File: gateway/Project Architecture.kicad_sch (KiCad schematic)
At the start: 0 parts

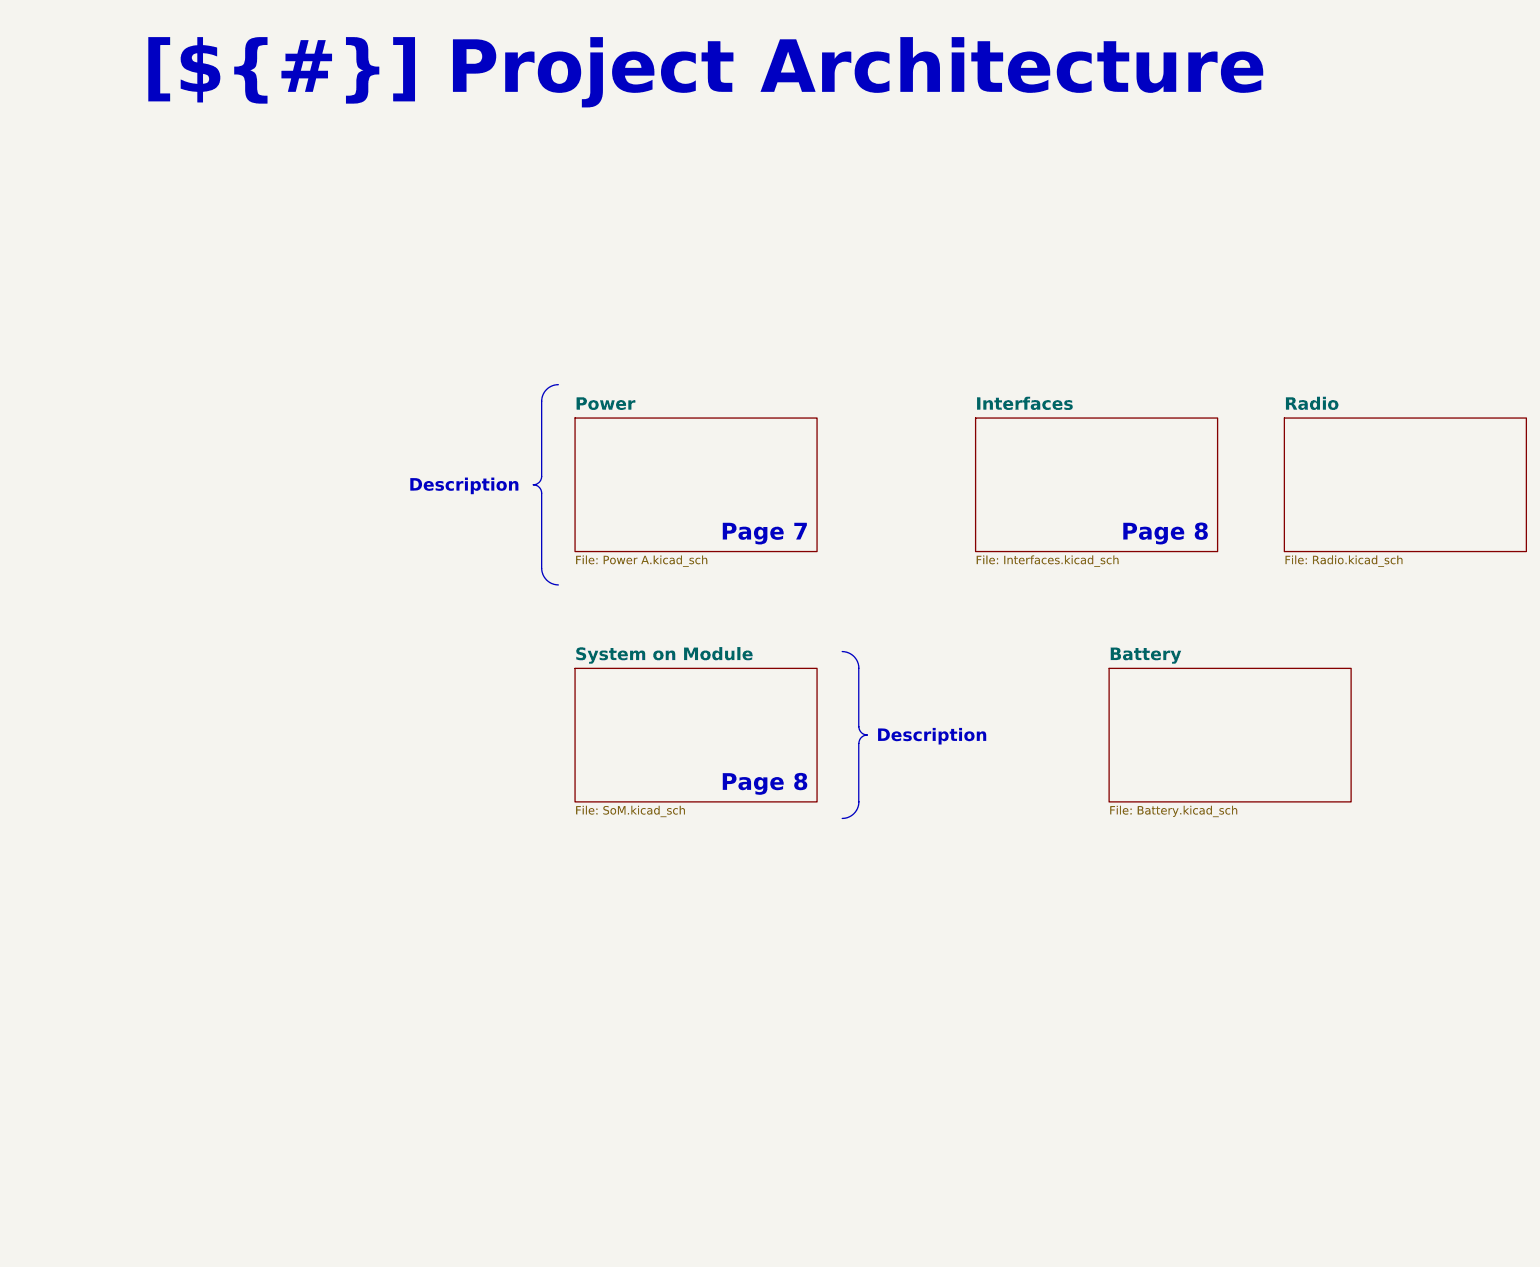
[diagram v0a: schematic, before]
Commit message: Working on first version
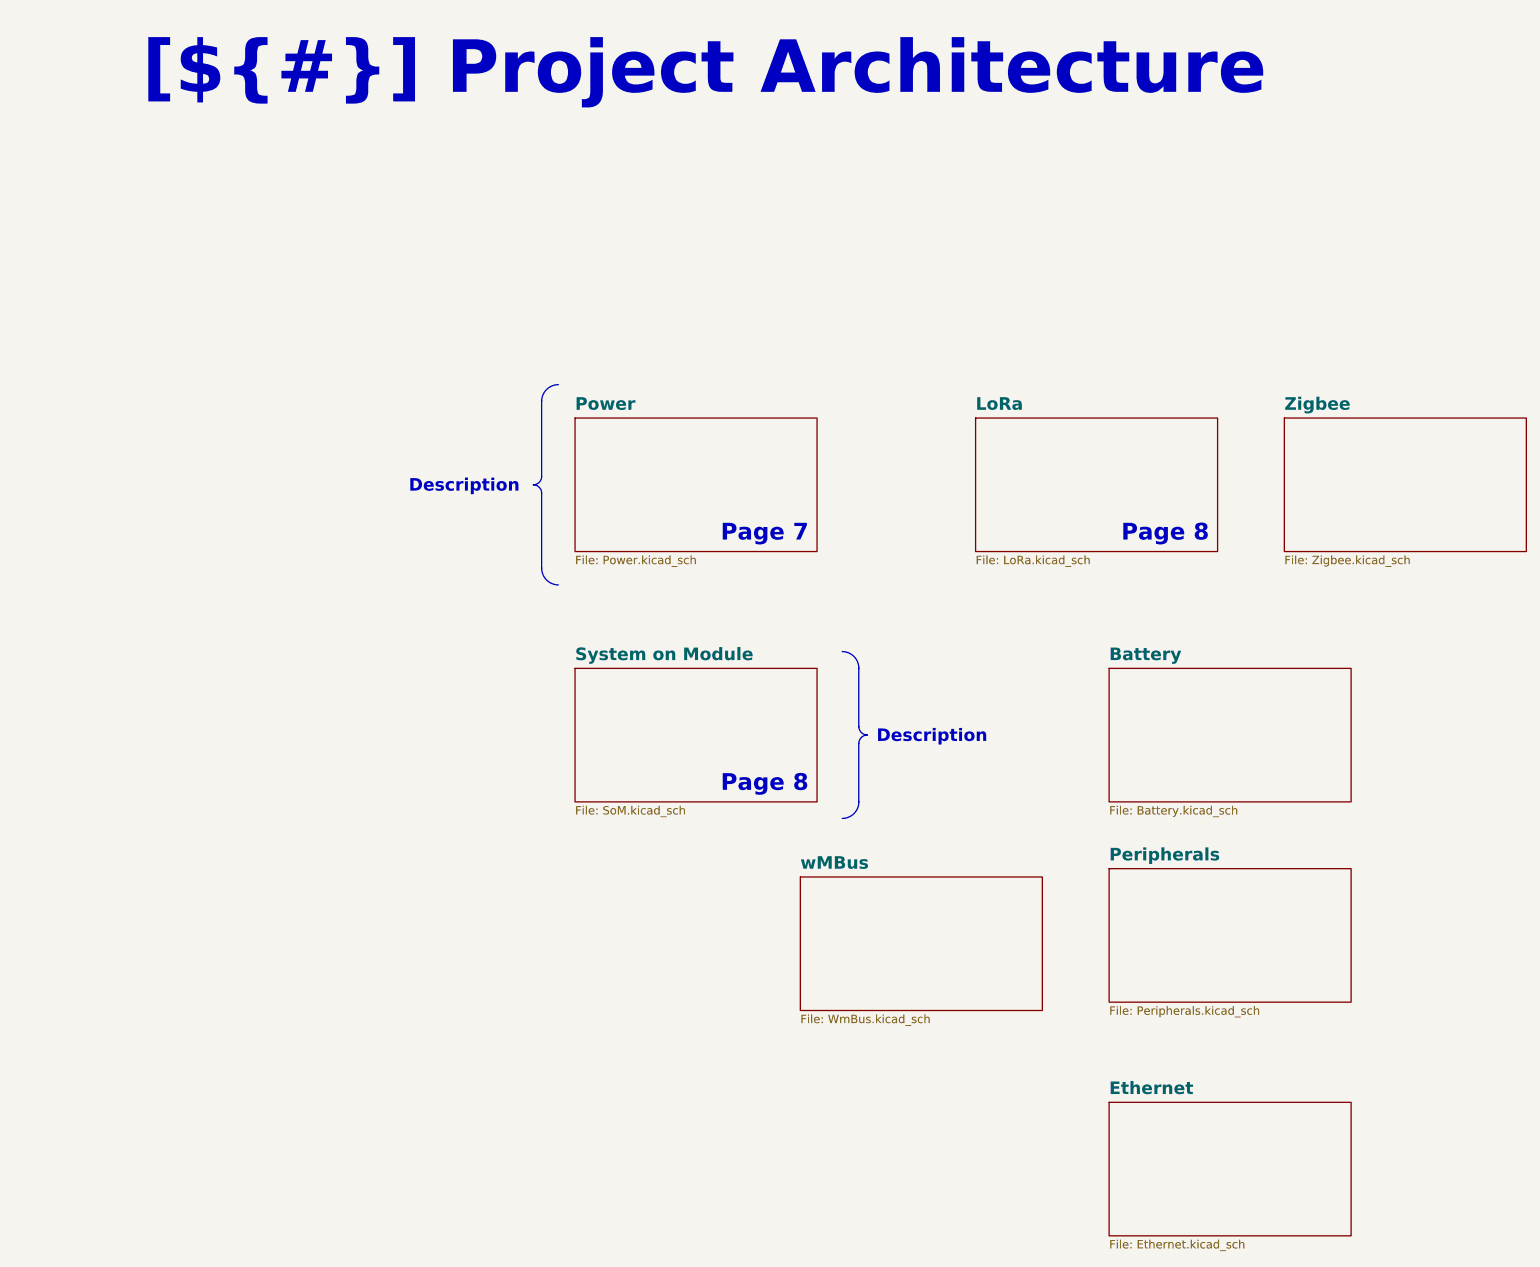
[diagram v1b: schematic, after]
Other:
- sheet Interfaces renamed LoRa
- sheet Radio renamed Zigbee
- added sheet Ethernet (Ethernet.kicad_sch)
- added sheet Peripherals (Peripherals.kicad_sch)
- added sheet wMBus (WmBus.kicad_sch)
- sheet LoRa: file Interfaces.kicad_sch -> LoRa.kicad_sch
- sheet Power: file Power A.kicad_sch -> Power.kicad_sch
- sheet Zigbee: file Radio.kicad_sch -> Zigbee.kicad_sch
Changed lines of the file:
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@@
 			(color 255 200 0 0.502)
 		)
-		(property "Sheetname" "Interfaces"
+		(property "Sheetname" "LoRa"
 			(at 251.46 75.1709 0)
 			(show_name no)
@@
 			)
 		)
-		(property "Sheetfile" "Interfaces.kicad_sch"
+		(property "Sheetfile" "LoRa.kicad_sch"
 			(at 251.46 97.1046 0)
 			(show_name no)
@@
 			(color 255 200 0 0.502)
 		)
-		(property "Sheetname" "Radio"
+		(property "Sheetname" "Zigbee"
 			(at 298.45 75.1709 0)
 			(show_name no)
@@
 			)
 		)
-		(property "Sheetfile" "Radio.kicad_sch"
+		(property "Sheetfile" "Zigbee.kicad_sch"
 			(at 298.45 97.1046 0)
 			(show_name no)
@@
 				(path "/d5742f03-3b1a-42e5-a384-018bd4b919aa/c5103ceb-5325-4a84-a025-9638a412984e"
 					(page "10")
+				)
+			)
+		)
+	)
+	(sheet
+		(at 224.79 146.05)
+		(size 36.83 20.32)
+		(exclude_from_sim no)
+		(in_bom yes)
+		(on_board yes)
+		(dnp no)
+		(fields_autoplaced yes)
+		(stroke
+			(width 0.1524)
+			(type solid)
+		)
+		(fill
+			(color 255 200 0 0.502)
+		)
+		(property "Sheetname" "wMBus"
+			(at 224.79 145.0209 0)
+			(show_name no)
+			(do_not_autoplace no)
+			(effects
+				(font
+					(size 1.905 1.905)
+					(bold yes)
+				)
+				(justify left bottom)
+			)
+		)
+		(property "Sheetfile" "WmBus.kicad_sch"
+			(at 224.79 166.9546 0)
+			(show_name no)
+			(do_not_autoplace no)
+			(effects
+				(font
+					(face "Arial")
+					(size 1.27 1.27)
+				)
+				(justify left top)
+			)
+		)
+		(instances
+			(project "Gateway"
+				(path "/d5742f03-3b1a-42e5-a384-018bd4b919aa/c5103ceb-5325-4a84-a025-9638a412984e"
+					(page "12")
+				)
+			)
+		)
+	)
+	(sheet
+		(at 271.78 144.78)
+		(size 36.83 20.32)
+		(exclude_from_sim no)
+		(in_bom yes)
+		(on_board yes)
+		(dnp no)
+		(fields_autoplaced yes)
+		(stroke
+			(width 0.1524)
+			(type solid)
+		)
+		(fill
+			(color 255 200 0 0.502)
+		)
+		(property "Sheetname" "Peripherals"
+			(at 271.78 143.7509 0)
+			(show_name no)
+			(do_not_autoplace no)
+			(effects
+				(font
+					(size 1.905 1.905)
+					(bold yes)
+				)
+				(justify left bottom)
+			)
+		)
+		(property "Sheetfile" "Peripherals.kicad_sch"
+			(at 271.78 165.6846 0)
+			(show_name no)
+			(do_not_autoplace no)
+			(effects
+				(font
+					(face "Arial")
+					(size 1.27 1.27)
+				)
+				(justify left top)
+			)
+		)
+		(instances
+			(project "Gateway"
+				(path "/d5742f03-3b1a-42e5-a384-018bd4b919aa/c5103ceb-5325-4a84-a025-9638a412984e"
+					(page "11")
+				)
+			)
+		)
+	)
+	(sheet
+		(at 271.78 180.34)
+		(size 36.83 20.32)
+		(exclude_from_sim no)
+		(in_bom yes)
+		(on_board yes)
+		(dnp no)
+		(fields_autoplaced yes)
+		(stroke
+			(width 0.1524)
+			(type solid)
+		)
+		(fill
+			(color 255 200 0 0.502)
+		)
+		(property "Sheetname" "Ethernet"
+			(at 271.78 179.3109 0)
+			(show_name no)
+			(do_not_autoplace no)
+			(effects
+				(font
+					(size 1.905 1.905)
+					(bold yes)
+				)
+				(justify left bottom)
+			)
+		)
+		(property "Sheetfile" "Ethernet.kicad_sch"
+			(at 271.78 201.2446 0)
+			(show_name no)
+			(do_not_autoplace no)
+			(effects
+				(font
+					(face "Arial")
+					(size 1.27 1.27)
+				)
+				(justify left top)
+			)
+		)
+		(instances
+			(project "Gateway"
+				(path "/d5742f03-3b1a-42e5-a384-018bd4b919aa/c5103ceb-5325-4a84-a025-9638a412984e"
+					(page "13")
 				)
 			)
@@
 			)
 		)
-		(property "Sheetfile" "Power A.kicad_sch"
+		(property "Sheetfile" "Power.kicad_sch"
 			(at 190.5 97.1046 0)
 			(show_name no)
